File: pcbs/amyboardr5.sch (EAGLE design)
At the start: 153 parts, among them Q2 S8050, Q5 S8050, U1 PCM9211PT, U15 H11L1SR2M, U16 SPX3819, U2 ESP32­S2­SOLO, U3 SPX3819, U4 TL074CD, U6 HX3608, Y1 22.5792MHZ

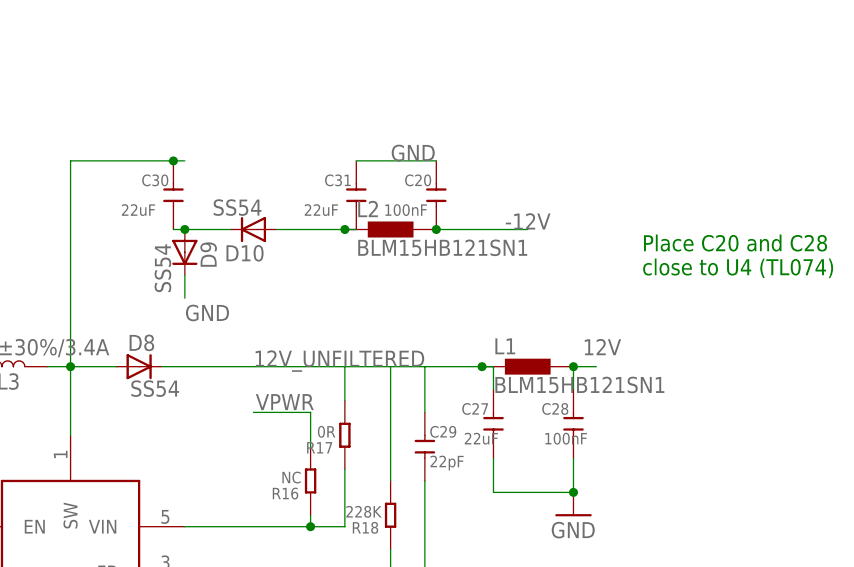
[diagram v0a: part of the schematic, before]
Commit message: copying usb fb
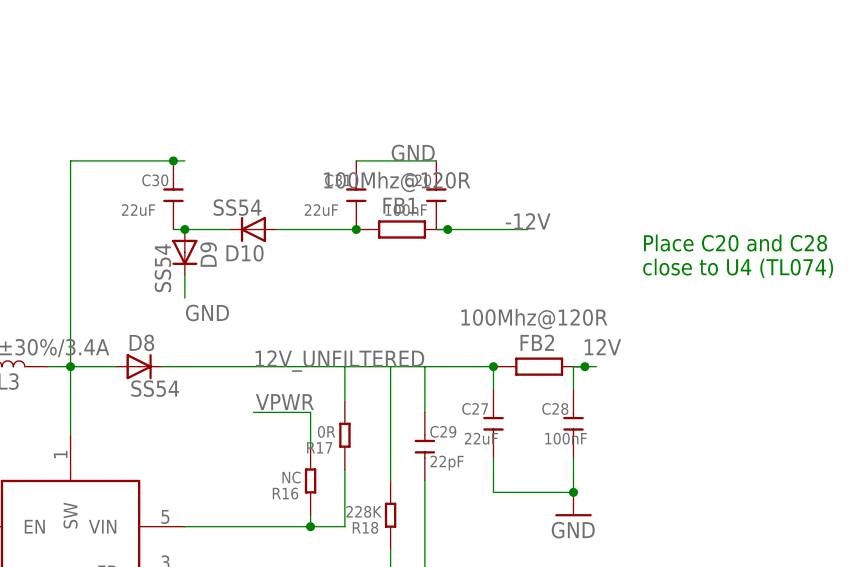
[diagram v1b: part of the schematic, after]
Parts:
- removed L1, L2: BLM15HB121SN1, inductors:BLM15HB121SN1
- added FB1, FB2: 100Mhz@120R, rcl:R-EU_R0805
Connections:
- net -12V: now also FB1.2; no longer L2.2
- net 12V: now also FB2.2; no longer L1.2
- net 12V_UNFILTERED: now also FB2.1; no longer L1.1
- net N$16: now also FB1.1; no longer L2.1
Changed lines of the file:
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@@
 <part name="R6" library="adafruit" deviceset="R-US_" device="R0805" value="10K"/>
 <part name="R8" library="adafruit" deviceset="R-US_" device="R0805" value="15K"/>
-<part name="L1" library="inductors" library_urn="urn:adsk.eagle:library:243" deviceset="BLM15H" device="" package3d_urn="urn:adsk.eagle:package:15132/1" technology="B121SN1"/>
-<part name="L2" library="inductors" library_urn="urn:adsk.eagle:library:243" deviceset="BLM15H" device="" package3d_urn="urn:adsk.eagle:package:15132/1" technology="B121SN1"/>
+<part name="FB1" library="rcl" deviceset="R-EU_" device="R0805" value="100Mhz@120R"/>
+<part name="FB2" library="rcl" deviceset="R-EU_" device="R0805" value="100Mhz@120R"/>
 </parts>
 <sheets>
@@
 <attribute name="VALUE" x="-99.06" y="-28.702" size="1.016" layer="96" font="vector" ratio="15" rot="R270"/>
 </instance>
-<instance part="L1" gate="G$1" x="287.02" y="-5.08" smashed="yes">
-<attribute name="NAME" x="283.21" y="-3.7084" size="1.778" layer="95"/>
-<attribute name="VALUE" x="283.21" y="-8.001" size="1.778" layer="96"/>
-</instance>
-<instance part="L2" gate="G$1" x="271.78" y="10.16" smashed="yes">
-<attribute name="NAME" x="267.97" y="11.5316" size="1.778" layer="95"/>
-<attribute name="VALUE" x="267.97" y="7.239" size="1.778" layer="96"/>
+<instance part="FB1" gate="G$1" x="273.05" y="10.16" smashed="yes">
+<attribute name="NAME" x="270.764" y="11.9126" size="1.778" layer="95"/>
+<attribute name="VALUE" x="264.16" y="14.732" size="1.778" layer="96"/>
+</instance>
+<instance part="FB2" gate="G$1" x="288.29" y="-5.08" smashed="yes">
+<attribute name="NAME" x="286.004" y="-3.3274" size="1.778" layer="95"/>
+<attribute name="VALUE" x="279.4" y="-0.508" size="1.778" layer="96"/>
 </instance>
 </instances>
@@
 <label x="284.48" y="10.16" size="1.778" layer="95"/>
 <pinref part="C20" gate="C" pin="2"/>
-<wire x1="276.86" y1="10.16" x2="287.02" y2="10.16" width="0.1524" layer="91"/>
-<pinref part="L2" gate="G$1" pin="2"/>
-<junction x="276.86" y="10.16"/>
+<wire x1="276.86" y1="10.16" x2="278.13" y2="10.16" width="0.1524" layer="91"/>
+<pinref part="FB1" gate="G$1" pin="2"/>
+<wire x1="278.13" y1="10.16" x2="287.02" y2="10.16" width="0.1524" layer="91"/>
+<junction x="278.13" y="10.16"/>
 </segment>
 <segment>
@@
 <segment>
 <pinref part="C28" gate="C" pin="1"/>
-<wire x1="292.1" y1="-5.08" x2="294.64" y2="-5.08" width="0.1524" layer="91"/>
+<wire x1="292.1" y1="-5.08" x2="293.37" y2="-5.08" width="0.1524" layer="91"/>
+<wire x1="293.37" y1="-5.08" x2="294.64" y2="-5.08" width="0.1524" layer="91"/>
 <wire x1="292.1" y1="-5.08" x2="292.1" y2="-7.62" width="0.1524" layer="91"/>
 <label x="293.116" y="-3.81" size="1.778" layer="95"/>
-<pinref part="L1" gate="G$1" pin="2"/>
-<junction x="292.1" y="-5.08"/>
+<pinref part="FB2" gate="G$1" pin="2"/>
+<junction x="293.37" y="-5.08"/>
 </segment>
 </net>
@@
 <pinref part="C31" gate="C" pin="2"/>
 <pinref part="D10" gate="G$1" pin="A"/>
-<wire x1="259.08" y1="10.16" x2="266.7" y2="10.16" width="0.1524" layer="91"/>
-<pinref part="L2" gate="G$1" pin="1"/>
-<wire x1="266.7" y1="10.16" x2="267.97" y2="10.16" width="0.1524" layer="91"/>
-<junction x="266.7" y="10.16"/>
+<wire x1="259.08" y1="10.16" x2="267.97" y2="10.16" width="0.1524" layer="91"/>
+<pinref part="FB1" gate="G$1" pin="1"/>
+<junction x="267.97" y="10.16"/>
 </segment>
 </net>
 <net name="12V_UNFILTERED" class="0">
 <segment>
-<pinref part="L1" gate="G$1" pin="1"/>
-<wire x1="281.94" y1="-5.08" x2="283.21" y2="-5.08" width="0.1524" layer="91"/>
 <pinref part="C27" gate="C" pin="1"/>
 <wire x1="283.21" y1="-7.62" x2="283.21" y2="-5.08" width="0.1524" layer="91"/>
 <pinref part="D8" gate="G$1" pin="C"/>
-<wire x1="246.38" y1="-5.08" x2="281.94" y2="-5.08" width="0.1524" layer="91"/>
-<junction x="281.94" y="-5.08"/>
+<wire x1="246.38" y1="-5.08" x2="283.21" y2="-5.08" width="0.1524" layer="91"/>
 <label x="256.54" y="-5.08" size="1.778" layer="95"/>
+<pinref part="FB2" gate="G$1" pin="1"/>
+<junction x="283.21" y="-5.08"/>
 </segment>
 <segment>
